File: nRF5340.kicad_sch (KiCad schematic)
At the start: 41 parts, among them SW1 BGS12P2L6, U2 nRF5340-CLXX, Y1 32.768KHz, Y1 32MHz

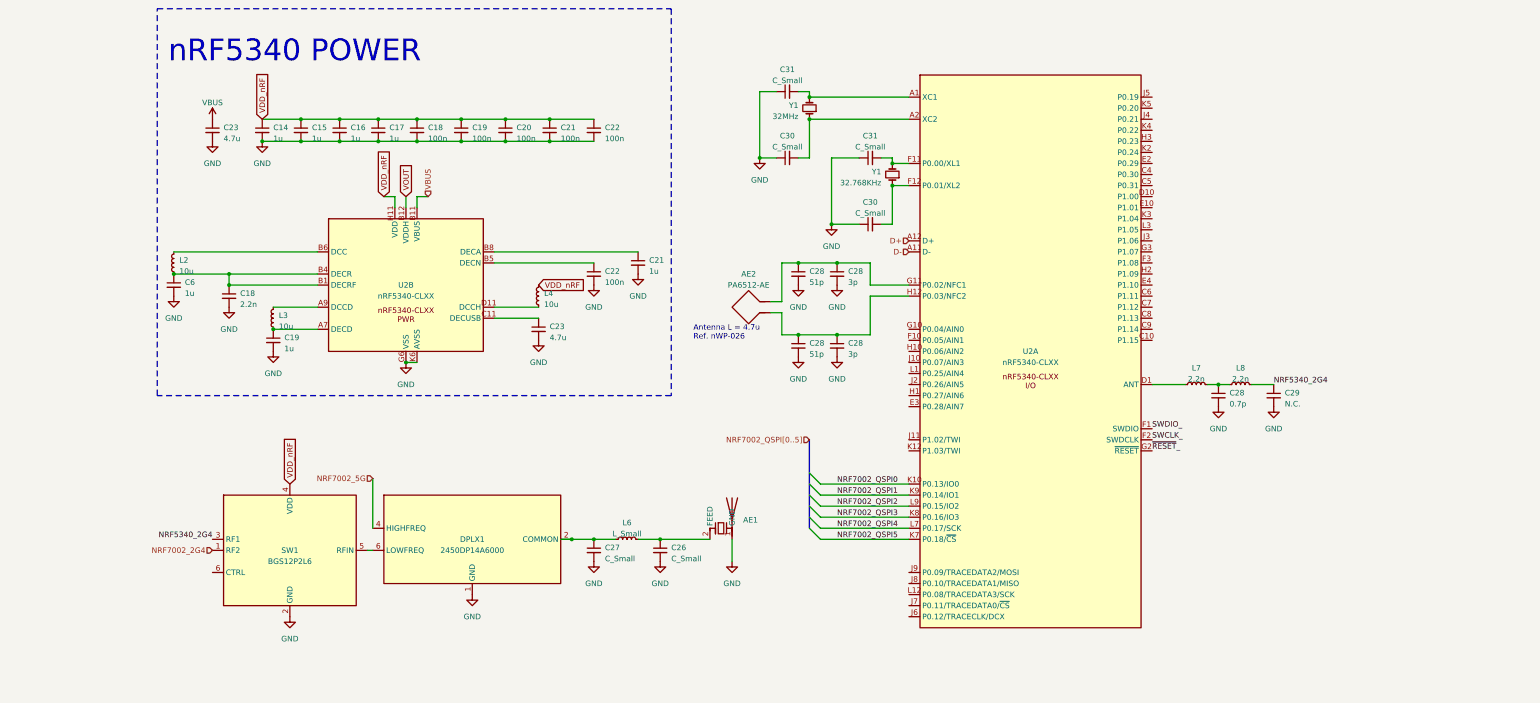
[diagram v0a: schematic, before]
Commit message: Schematic complete.
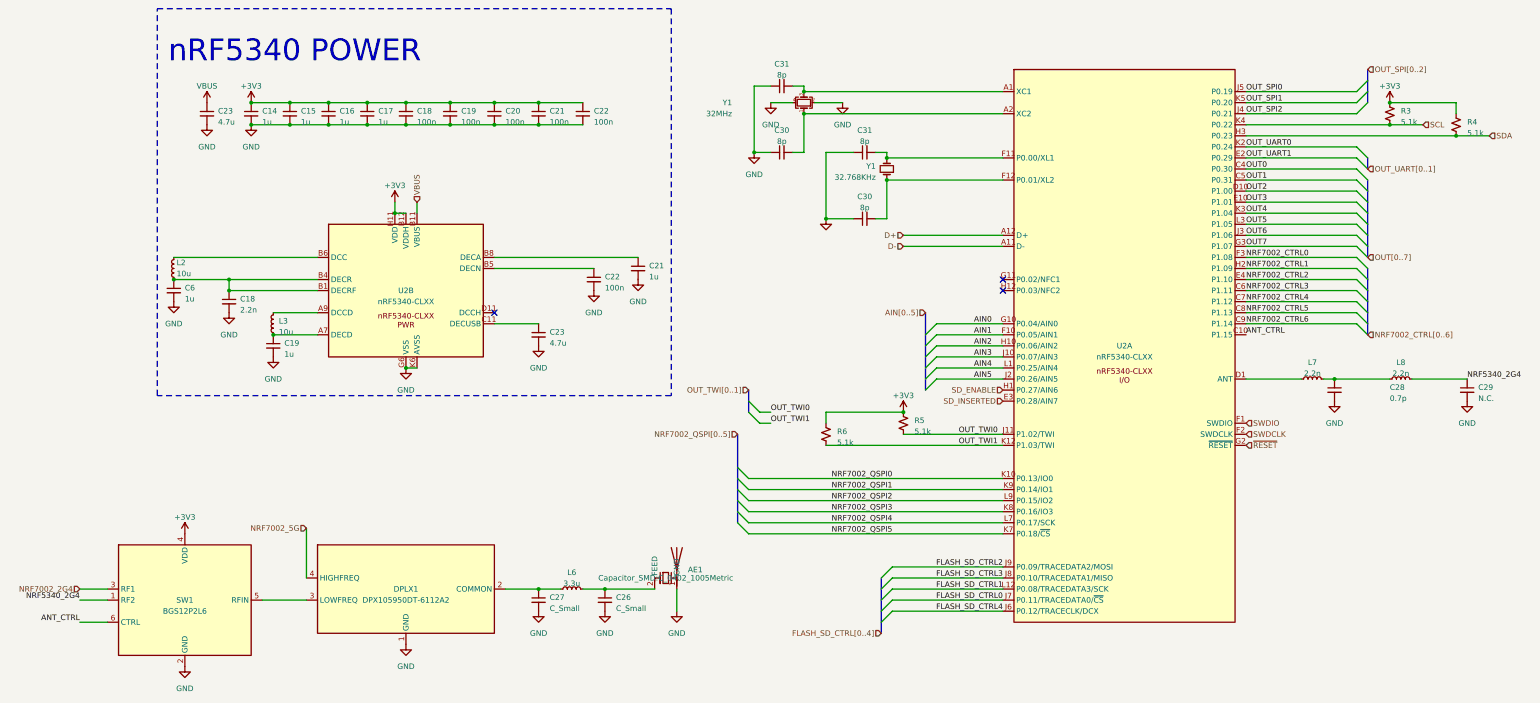
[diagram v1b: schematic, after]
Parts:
- removed AE2: PA6512-AE, symbol Device:Antenna_Loop
- removed C28 (x2): 3p, symbol Device:C_Small
- removed C28 (x2): 51p, symbol Device:C_Small
- removed DPLX1: 2450DP14A6000, rf-lib:2450DP14A6000, symbol rf-lib:2450DP14A6000
- removed L4: 10u, symbol Device:L_Small
- added DPLX1: DPX105950DT-6112A2, rf-lib:DPX105950DT-6112A2, symbol rf-lib:DPX105950DT-6112A2
- added R3, R4, R5, R6: 5.1k, Resistor_SMD:R_0603_1608Metric, symbol Device:R_Small_US
- AE1: value ~ -> Capacitor_SMD:C_0402_1005Metric; MPN (none) -> 2450AD14A5500
- C14, C15, C16, C17, C19, C21, C23, C6: footprint (none) -> Capacitor_SMD:C_0402_1005Metric
- C18, C19, C20, C21, C22, C26, C27, C28, C29: footprint (none) -> Capacitor_SMD:C_0201_0603Metric
- C30, C31: value C_Small -> 8p; footprint (none) -> Capacitor_SMD:C_0201_0603Metric
- L2, L3: footprint (none) -> Inductor_SMD:L_0603_1608Metric
- L6: value L_Small -> 3.3u; footprint (none) -> Inductor_SMD:L_0201_0603Metric
- L7, L8: footprint (none) -> Inductor_SMD:L_0201_0603Metric
- Y1: footprint (none) -> Crystal:Crystal_SMD_2016-4Pin_2.0x1.6mm; symbol Device:Crystal_Small -> Device:Crystal_GND24_Small; MPN (none) -> XRCGB32M000F1S1AR0
- Y1: footprint (none) -> Crystal:Crystal_SMD_3215-2Pin_3.2x1.5mm; MPN (none) -> ECS-.327-6-12-TR9
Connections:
- net VOUT is gone; now on net +3V3: U2.B12 (VDDH)
- net GND: now also Y1.2, Y1.4, DPLX1.1 (GND)
- net NRF5340_2G4: now also SW1.1 (RF2); no longer SW1.3 (RF1)
- net NRF7002_2G4: now also SW1.3 (RF1); no longer SW1.1 (RF2)
- net NRF7002_5G: now also DPLX1.4 (HIGHFREQ)
- net at C27.1, L6.1: now also DPLX1.2 (COMMON)
- net at SW1.5 (RFIN): now also DPLX1.3 (LOWFREQ)
- net at C31.2, U2.A1 (XC1): now also Y1.3; no longer Y1.2
- net ANT_CTRL: now reaches U2.C10 (P1.15)
- net ANT_CTRL: now also SW1.6 (CTRL)
- net OUT0: now reaches U2.C4 (P0.30)
- net OUT1: now reaches U2.C5 (P0.31)
- net NRF7002_CTRL3: now reaches U2.C6 (P1.11)
- net NRF7002_CTRL4: now reaches U2.C7 (P1.12)
- net NRF7002_CTRL5: now reaches U2.C8 (P1.13)
- net NRF7002_CTRL6: now reaches U2.C9 (P1.14)
- net OUT2: now reaches U2.D10 (P1.00)
- net OUT3: now reaches U2.E10 (P1.01)
- net OUT_UART1: now reaches U2.E2 (P0.29)
- net SD_INSERTED: now reaches U2.E3 (P0.28/AIN7)
- net NRF7002_CTRL2: now reaches U2.E4 (P1.10)
- net AIN1: now reaches U2.F10 (P0.05/AIN1)
- net NRF7002_CTRL0: now reaches U2.F3 (P1.08)
- net AIN0: now reaches U2.G10 (P0.04/AIN0)
- net OUT7: now reaches U2.G3 (P1.07)
- net SD_ENABLE: now reaches U2.H1 (P0.27/AIN6)
- net AIN2: now reaches U2.H10 (P0.06/AIN2)
- net NRF7002_CTRL1: now reaches U2.H2 (P1.09)
- net SDA: now reaches U2.H3 (P0.23)
- net SDA: now also R4.2
- net AIN3: now reaches U2.J10 (P0.07/AIN3)
- net OUT_TWI0: now reaches U2.J11 (P1.02/TWI)
- net OUT_TWI0: now also R5.2
- net AIN5: now reaches U2.J2 (P0.26/AIN5)
- net OUT6: now reaches U2.J3 (P1.06)
- net OUT_SPI2: now reaches U2.J4 (P0.21)
- net OUT_SPI0: now reaches U2.J5 (P0.19)
- net FLASH_SD_CTRL4: now reaches U2.J6 (P0.12/TRACECLK/DCX)
- net FLASH_SD_CTRL0: now reaches U2.J7 (P0.11/TRACEDATA0/~{CS})
- net FLASH_SD_CTRL3: now reaches U2.J8 (P0.10/TRACEDATA1/MISO)
- net FLASH_SD_CTRL2: now reaches U2.J9 (P0.09/TRACEDATA2/MOSI)
- net OUT_TWI1: now reaches U2.K12 (P1.03/TWI)
- net OUT_TWI1: now also R6.2
- net OUT_UART0: now reaches U2.K2 (P0.24)
- net OUT4: now reaches U2.K3 (P1.04)
- net SCL: now reaches U2.K4 (P0.22)
- net SCL: now also R3.2
- net OUT_SPI1: now reaches U2.K5 (P0.20)
- net AIN4: now reaches U2.L1 (P0.25/AIN4)
- net FLASH_SD_CTRL1: now reaches U2.L12 (P0.08/TRACEDATA3/SCK)
- net OUT5: now reaches U2.L3 (P1.05)
- net SWCLK_ renamed SWDCLK
- net SWDIO_ renamed SWDIO
- net VDD_nRF renamed +3V3
- net +3V3: now also R3.1, R4.1, R5.1, R6.1
- net ~{RESET}_ renamed ~{RESET}
- no-connect marks 0 -> 3
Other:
- note removed: "Antenna L = 4.7u Ref. nWP-026"
- moved on the sheet: AE1, C14, C15, C16, C17, C18, C19, C20, C21, C22, C23, C26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
